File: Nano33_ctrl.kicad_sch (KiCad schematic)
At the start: 52 parts, among them J1 To Protec_Brd, J12 Conn_01x02, J15 To Display, J17 Conn_01x02, J18 To Protec_Brd encoder, J19 To P.A., J4 Power_In, J5 Conn_01x02, J6 Conn_01x02, U12 Arduino-NANO-33, U2 LM1117S-5.0, U3 LM1117S-3.3, U4 74HCT04, U5 TPIC6595, U6 TPIC6595, U7 TPIC6595, U8 24FC1025-I_SN, U9 24FC1025-I_SN

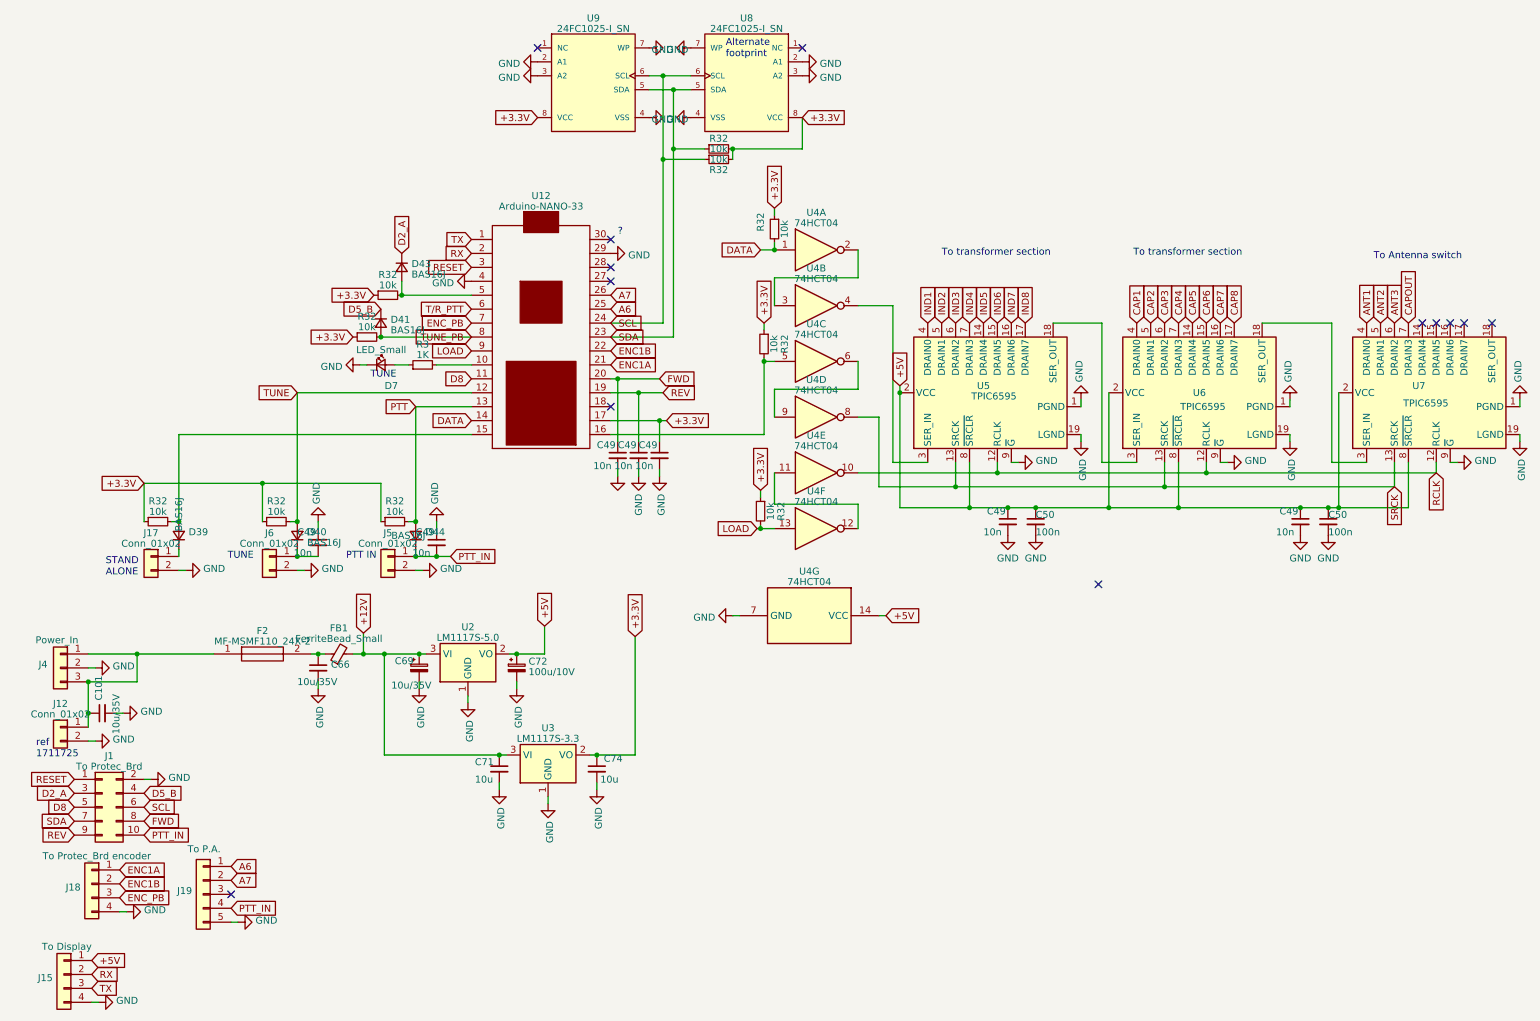
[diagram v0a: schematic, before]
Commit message: intermediate git, more traces to come
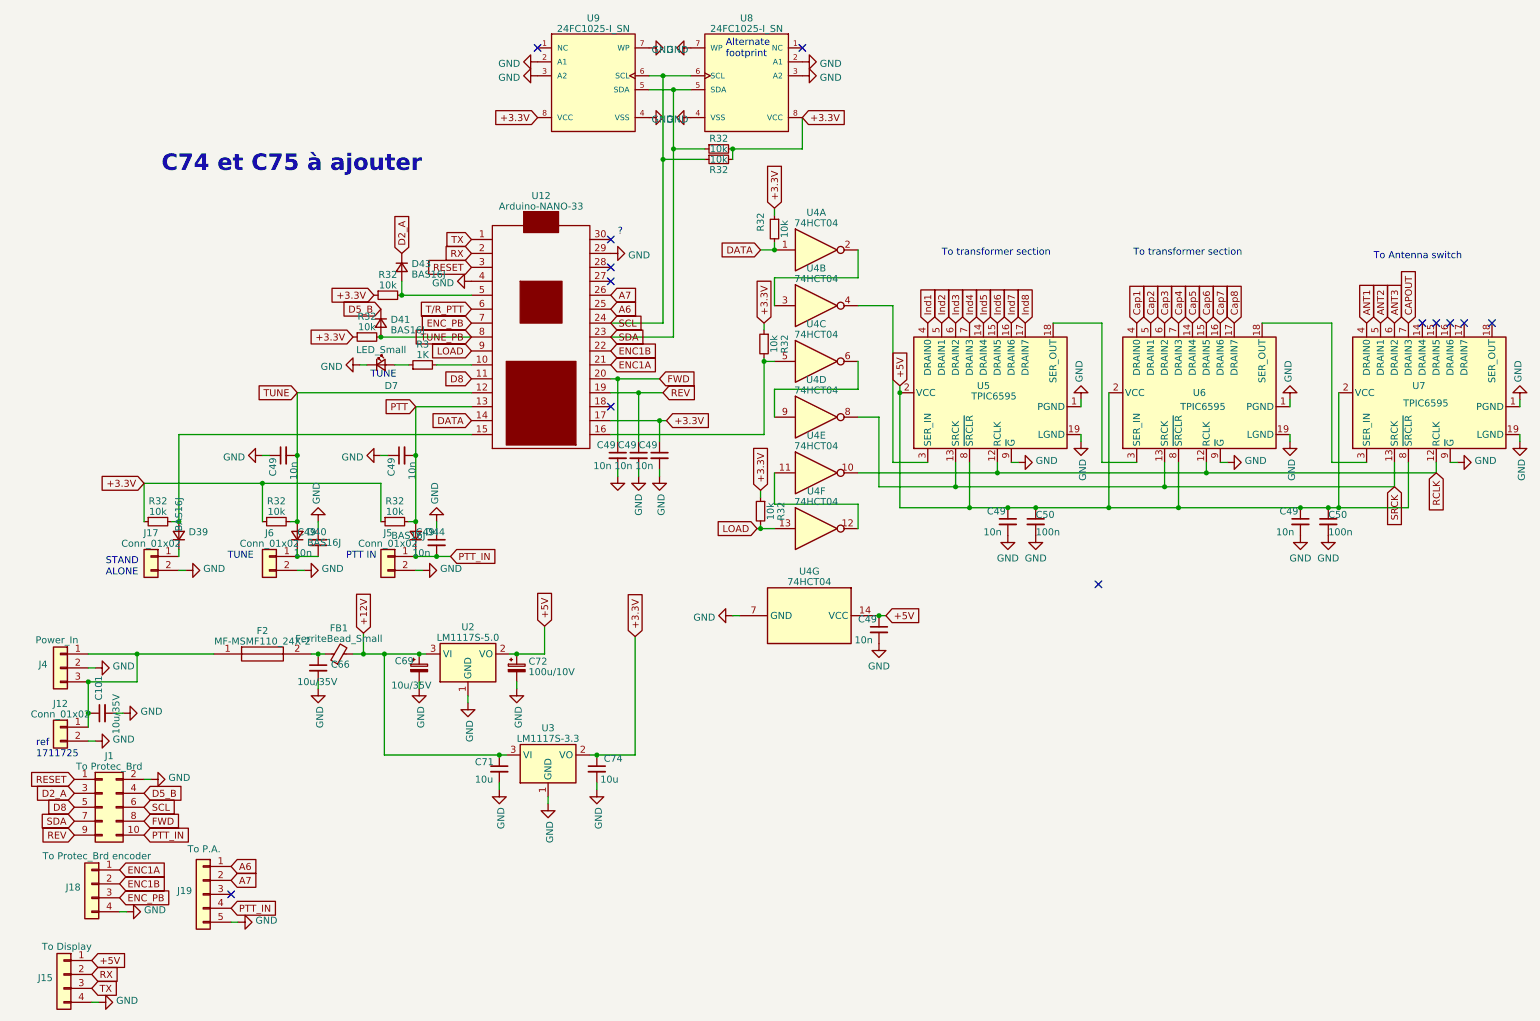
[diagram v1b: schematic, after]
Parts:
- added C49 (x3): 10n, Capacitor_SMD:C_0805_2012Metric_Pad1.18x1.45mm_HandSolder, symbol Device:C_Small
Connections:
- net +5V: now also C49.1
- net GND: now also C49.1, C49.1, C49.2
- net PTT: now also C49.2
- net TUNE: now also C49.2
- net CAP1 renamed Cap1
- net CAP2 renamed Cap2
- net CAP3 renamed Cap3
- net CAP4 renamed Cap4
- net CAP5 renamed Cap5
- net CAP6 renamed Cap6
- net CAP7 renamed Cap7
- net CAP8 renamed Cap8
- net IND1 renamed Ind1
- net IND2 renamed Ind2
- net IND3 renamed Ind3
- net IND4 renamed Ind4
- net IND5 renamed Ind5
- net IND6 renamed Ind6
- net IND7 renamed Ind7
- net IND8 renamed Ind8
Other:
- note added: "C74 et C75 à ajouter"
